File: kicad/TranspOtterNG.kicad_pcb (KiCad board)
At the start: 2 copper layers, 90.6 x 38.1 mm, 51 parts, among them J1 UART/I2C, J2 UART/IO/ANALOG, J8 Conn_01x05_Male, U1 AMS1117, U2 LM2596S-5

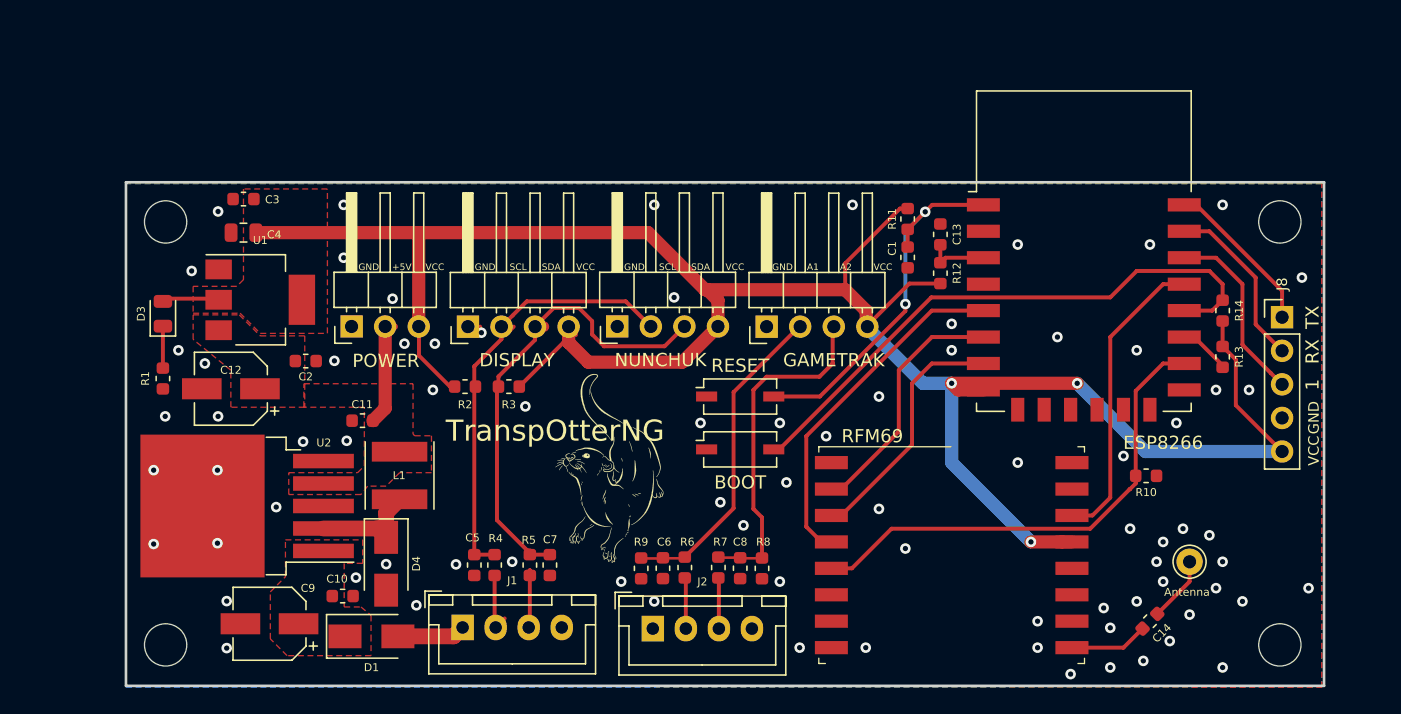
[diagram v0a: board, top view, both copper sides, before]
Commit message: minor changes, now v2
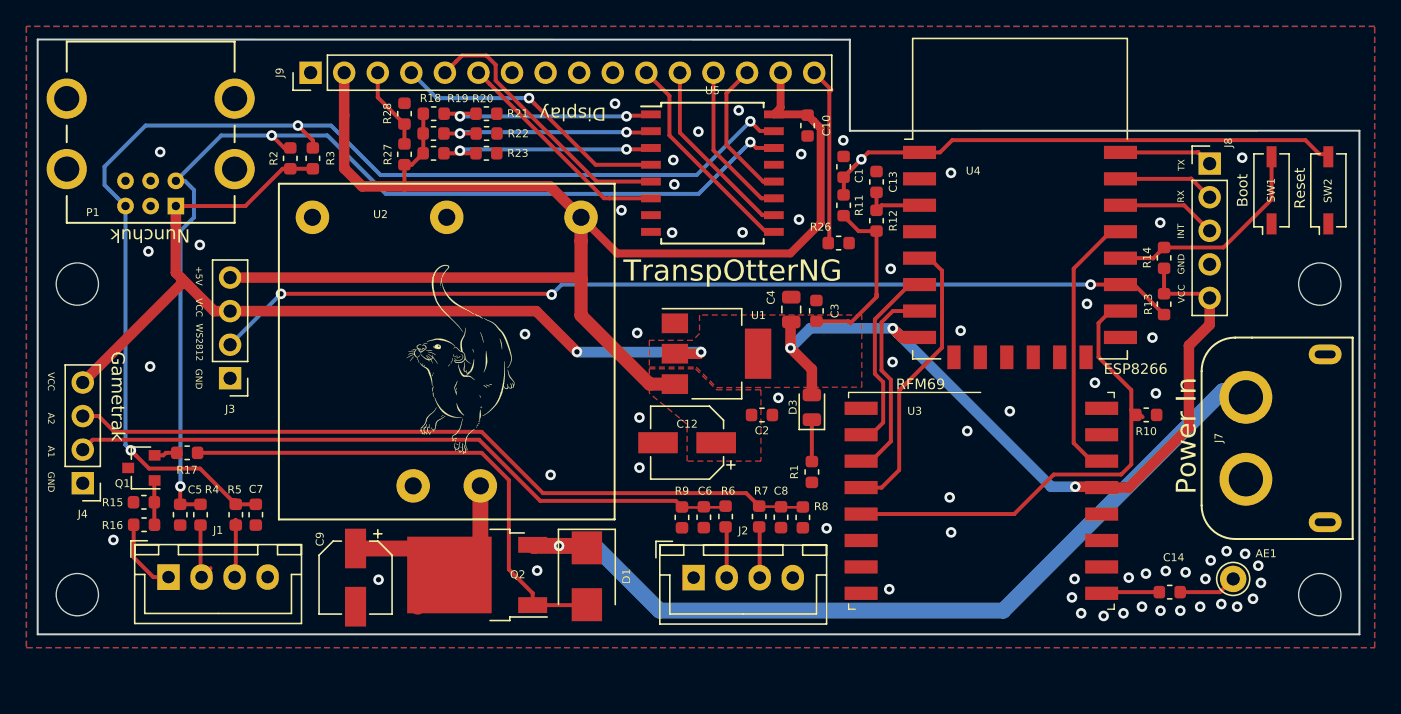
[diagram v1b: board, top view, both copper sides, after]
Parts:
- removed Antenna: Antenna, Connector_Pin:Pin_D1.0mm_L10.0mm
- removed BOOT: Flash, Button_Switch_SMD:SW_DIP_SPSTx01_Slide_Copal_CHS-01A_W5.08mm_P1.27mm_JPin
- removed C11: 100n, Capacitor_SMD:C_0603_1608Metric
- removed D4: 1N5822, Diode_SMD:D_SMA
- removed DISPLAY: Display, Connector_PinHeader_2.54mm:PinHeader_1x04_P2.54mm_Horizontal
- removed ESP8266: ESP-12E, RF_Module:ESP-12E
- removed GAMETRAK: GameTrak, Connector_PinHeader_2.54mm:PinHeader_1x04_P2.54mm_Horizontal
- removed L1: L, Inductor_SMD:L_Taiyo-Yuden_MD-5050
- removed NUNCHUK: Nunchuk, Connector_PinHeader_2.54mm:PinHeader_1x04_P2.54mm_Horizontal
- removed POWER: Power, Connector_PinHeader_2.54mm:PinHeader_1x03_P2.54mm_Horizontal
- removed RESET: Reset, Button_Switch_SMD:SW_DIP_SPSTx01_Slide_Copal_CHS-01A_W5.08mm_P1.27mm_JPin
- removed RFM69: RFM69HCW, RF_Module:HOPERF_RFM69HW
- added AE1: Antenna, Connector_Pin:Pin_D1.0mm_L10.0mm, F.Cu at (190.4, 80.8)
- added J3: Conn_01x04_Male, Connector_PinHeader_2.54mm:PinHeader_1x04_P2.54mm_Vertical, F.Cu at (114.6, 65.6)
- added J4: GameTrak, Connector_PinHeader_2.54mm:PinHeader_1x04_P2.54mm_Vertical, F.Cu at (103.4, 73.6)
- added J7: xt30, otter:XT60_angle, F.Cu at (194.4, 70.2)
- added J9: Conn_01x16_Female, Connector_PinHeader_2.54mm:PinHeader_1x16_P2.54mm_Vertical, F.Cu at (120.6, 42.5)
- added P1: CONN_WII, otter:CONN_WII, F.Cu at (108.5, 47.0)
- added Q1: Q_NMOS_GDS, Package_TO_SOT_SMD:SOT-23, F.Cu at (107.8, 72.4)
- added Q2: Q_PMOS_GDS, Package_TO_SOT_SMD:TO-252-2, F.Cu at (133.2, 80.5)
- added R15: 100k, Resistor_SMD:R_0603_1608Metric, F.Cu at (108.0, 76.7)
- added R16: 100k, Resistor_SMD:R_0603_1608Metric, F.Cu at (108.0, 75.0)
- added R17: 100k, Resistor_SMD:R_0603_1608Metric, F.Cu at (111.3, 71.3)
- added R18: 10k, Resistor_SMD:R_0603_1608Metric, F.Cu at (130.0, 45.6)
- added R19: 10k, Resistor_SMD:R_0603_1608Metric, F.Cu at (129.9, 47.1)
- added R20: 10k, Resistor_SMD:R_0603_1608Metric, F.Cu at (129.9, 48.6)
- added R21: DNP, Resistor_SMD:R_0603_1608Metric, F.Cu at (133.9, 45.6)
- added R22: DNP, Resistor_SMD:R_0603_1608Metric, F.Cu at (134.0, 47.1)
- added R23: DNP, Resistor_SMD:R_0603_1608Metric, F.Cu at (133.9, 48.6)
- added R26: 220, Resistor_SMD:R_0603_1608Metric, F.Cu at (160.6, 55.4)
- added R27: 10k, Resistor_SMD:R_0603_1608Metric, F.Cu at (127.7, 48.7)
- added R28: 10k, Resistor_SMD:R_0603_1608Metric, F.Cu at (127.7, 45.6)
- added SW1: Flash, Button_Switch_SMD:SW_DIP_SPSTx01_Slide_Copal_CHS-01A_W5.08mm_P1.27mm_JPin, F.Cu at (193.3, 51.4)
- added SW2: Reset, Button_Switch_SMD:SW_DIP_SPSTx01_Slide_Copal_CHS-01A_W5.08mm_P1.27mm_JPin, F.Cu at (197.6, 51.4)
- added U3: RFM69HCW, RF_Module:HOPERF_RFM69HW, F.Cu at (171.4, 74.9)
- added U4: ESP-12E, RF_Module:ESP-12E, F.Cu at (174.3, 52.0)
- added U5: PCF8574, Package_SO:SOIC-16W_7.5x10.3mm_P1.27mm, F.Cu at (151.0, 50.1)
- C12, C9: value 470u -> 20u
- D1: value 1N4001 -> 12V; footprint Diode_SMD:D_SMA -> Diode_SMD:D_SMB
- U2: value LM2596S-5 -> URB4805YMD-6WR3; footprint Package_TO_SOT_SMD:TO-263-5_TabPin3 -> otter:URB4805YMD-6WR3
- moved C10 50.0 mm to (158.2, 46.5), turned to 270 degrees
- moved D3 49.6 mm to (158.6, 67.8)
- moved R1 49.6 mm to (158.6, 72.7)
- moved C3 44.2 mm to (158.9, 60.5), turned to 90 degrees
- moved C4 41.9 mm to (157.0, 60.4), turned to 90 degrees
- moved C12 34.8 mm to (149.1, 70.5)
- moved C2 34.8 mm to (154.8, 68.4)
- moved U1 34.8 mm to (151.4, 63.8)
- moved R3 22.8 mm to (120.8, 49.0), turned to 90 degrees
- moved J1 22.6 mm to (109.9, 80.7)
- moved C5 22.6 mm to (110.8, 76.0)
- moved C7 22.6 mm to (116.5, 76.0)
- moved R4 22.6 mm to (112.3, 76.0)
- moved R5 22.6 mm to (115.0, 76.0)
- moved R2 21.8 mm to (119.1, 49.0), turned to 90 degrees
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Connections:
- C10 pad 1: +15V -> +5V
- C9 pad 1: +15V -> Net-(C9-Pad1)
- D1 pad 1: +15V -> Net-(D1-Pad1)
- J1 pad 1: Net-(D1-Pad2) -> +15V
- R13 pad 2: Net-(R13-Pad2) -> WS2812
- U2 pad 1: +15V -> GND
- U2 pad 2: Net-(D4-Pad1) -> Net-(C9-Pad1)
- U2 pad 3: GND -> +5V
- U2 pad 4: +5V -> (no net)
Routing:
- net +5V: track 7.90 -> 111.3 mm
- net WS2812: track 0.00 -> 74.3 mm, vias 0 -> 3
- net Net-(D1-Pad1): track 0.00 -> 67.0 mm, vias 0 -> 1
- net RX0_SDA: track 35.1 -> 91.3 mm, vias 0 -> 3
- net TX0_SCL: track 33.7 -> 79.6 mm, vias 0 -> 3
- net Net-(D1-Pad2): track 5.17 -> 38.7 mm
- net RX1_ADC2: track 25.9 -> 57.3 mm
- net GPIO0: track 44.4 -> 16.5 mm
- net TX1_ADC1: track 24.3 -> 51.1 mm
- net VCC: track 173.3 -> 148.4 mm, vias 3 -> 5
- net RS: track 0.00 -> 21.0 mm, vias 0 -> 1
- net RW: track 0.00 -> 20.8 mm
- net Net-(C9-Pad1): track 0.00 -> 19.0 mm
- net CS: track 0.00 -> 17.1 mm
- net A2: track 0.00 -> 16.7 mm, vias 0 -> 2
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- removed copper zone on F.Cu, net +15V
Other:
- board size 90.6 x 38.1 mm -> 100 x 45 mm
- board text added: "Boot"
- board text added: "Display"
- board text added: "ESP8266"
- board text added: "Gametrak"
- board text added: "INT"
- board text added: "Nunchuk"
- board text added: "Power In"
- board text added: "RFM69"
- board text added: "Reset"
- board text added: "WS2812"
- board text removed: "1"
- board text removed: "SCL"
- board text removed: "SDA"
